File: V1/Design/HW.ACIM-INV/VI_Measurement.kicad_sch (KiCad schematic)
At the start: 59 parts, among them Q1 20V/1A, U12 OP-1CH, U15 OP-1CH, U16 OP-1CH, U2 OP-1CH, U4 CMP-1CH

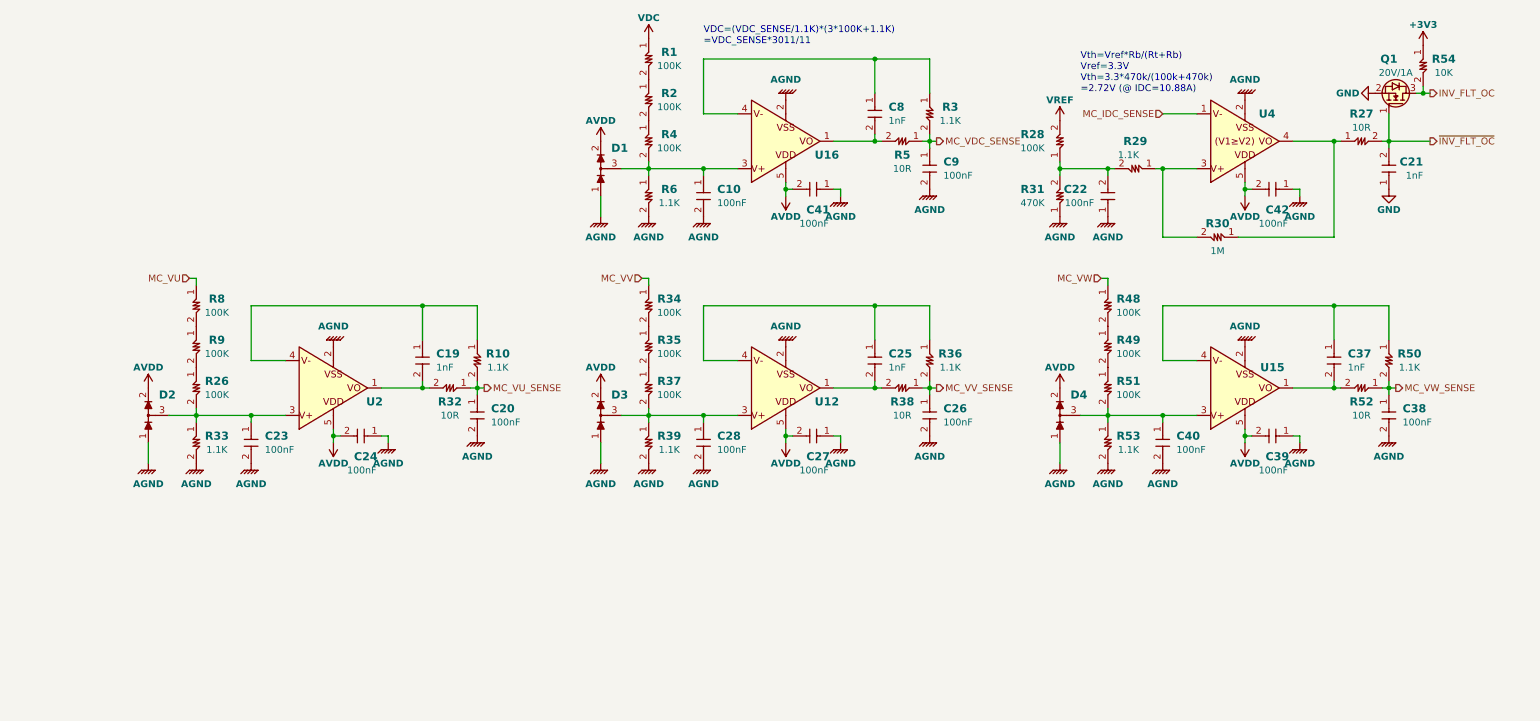
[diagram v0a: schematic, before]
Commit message: V1 schematic update 2
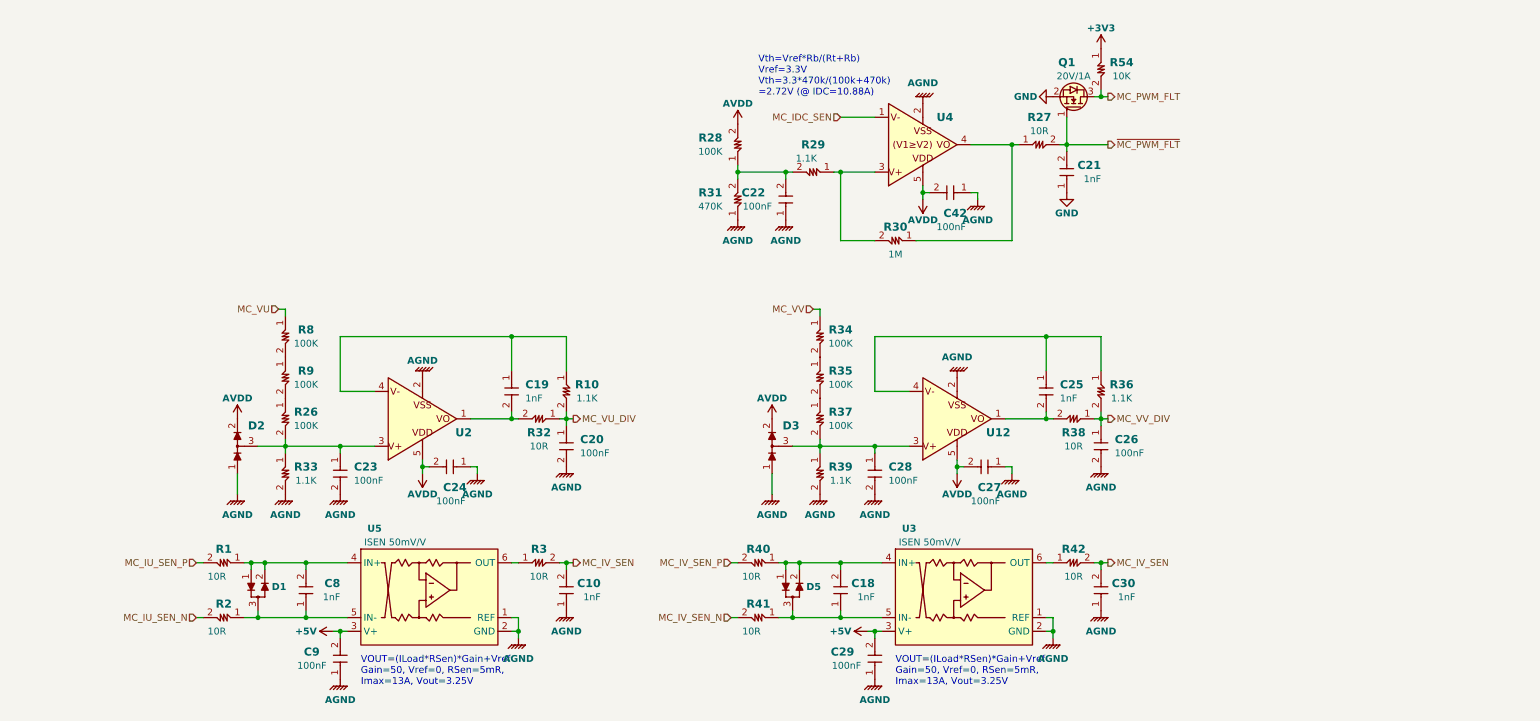
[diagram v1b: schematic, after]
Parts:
- removed C37: 1nF, SAMPI:CAP0603, symbol SAMPI:CERCAP
- removed C38, C39, C40, C41: 100nF, SAMPI:CAP0603, symbol SAMPI:CERCAP
- removed D1, D4: GP DIODE, SAMPI:SOT23, symbol SAMPI:DIODE_ARR2
- removed R4, R48, R49, R51: 100K, SAMPI:RES0603, symbol SAMPI:RES
- removed R5, R52: 10R, SAMPI:RES0603, symbol SAMPI:RES
- removed R50, R53, R6: 1.1K, SAMPI:RES0603, symbol SAMPI:RES
- removed U15, U16: OP-1CH, SAMPI:SOT353, symbol SAMPI:OPAMP-1CH
- added C18, C30: 1nF, SAMPI:CAP0603, symbol SAMPI:CERCAP
- added C29: 100nF, SAMPI:CAP0603, symbol SAMPI:CERCAP
- added D1, D5: GP DIODE, SAMPI:SOT23, symbol SAMPI:DIODE_ARR1
- added R40, R41, R42: 10R, SAMPI:RES0603, symbol SAMPI:RES
- added U3, U5: ISEN 50mV/V, SAMPI:SOT363, symbol SAMPI:ZXCT199Q
- C10: value 100nF -> 1nF; MNP CL10B104KB8NNNC -> CL10B102KB8NNNC; Unit Price 0.0146 -> 0.027
- R1, R2: value 100K -> 10R; MNP RC0603FR-07100KL -> RC0603FR-0710RL; Unit Price 0.019 -> 0.029
- R3: value 1.1K -> 10R; MNP AC0603FR-071K1L -> RC0603FR-0710RL; Unit Price 0.021 -> 0.029
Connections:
- net VDC is gone; now on an unnamed net: R1.1
- net VREF is gone; now on net AVDD: R28.2
- net AGND: now also C10.1, C9.1, C29.1, C30.1, U3.1 (REF), U3.2 (GND), U5.1 (REF), U5.2 (GND); no longer C10.2, C9.2
- net at C8.1: now also R2.1, D1.3 (COM), U5.5 (IN-); no longer R3.1
- net MC_IU_SEN_N: now reaches R2.2
- net at C8.2: now also D1.1 (A1), D1.2 (K2), U5.4 (IN+)
- net MC_IU_SEN_P: now reaches R1.2
- net MC_IU_SEN_P: no longer R2.1
- net INV_FLT_OC renamed MC_PWM_FLT
- net MC_IDC_SENSE renamed MC_IDC_SEN
- net MC_VDC_SENSE renamed MC_IV_SEN
- net MC_IV_SEN: now also C10.2, C30.2, R42.2; no longer C9.1
- net MC_VU_SENSE renamed MC_VU_DIV
- net MC_VV_SENSE renamed MC_VV_DIV
- net ~{INV_FLT_OC} renamed ~{MC_PWM_FLT}
- new net: C18.1, D5.3 (COM), R41.1, U3.5 (IN-)
- new net: R42.1, U3.6 (OUT)
- new net: C18.2, D5.1 (A1), D5.2 (K2), R40.1, U3.4 (IN+)
- new net: R3.1, U5.6 (OUT)
- new net +5V: C29.2, C9.2, U3.3 (V+), U5.3 (V+)
- new net MC_IV_SEN_N: R41.2
- new net MC_IV_SEN_P: R40.2
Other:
- note added: "VOUT=(ILoad*RSen)*Gain+Vref Gain=50, Vref=0, RSen=5mR, Imax=13A, Vout=3.25V"
- note removed: "VDC=(VDC_SENSE/1.1K)*(3*100K+1.1K) =VDC_SENSE*3011/11"
- moved on the sheet: C19, C20, C21, C22, C23, C24, C25, C26, C27, C28, C42, D2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

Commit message: V1 schematic update 3
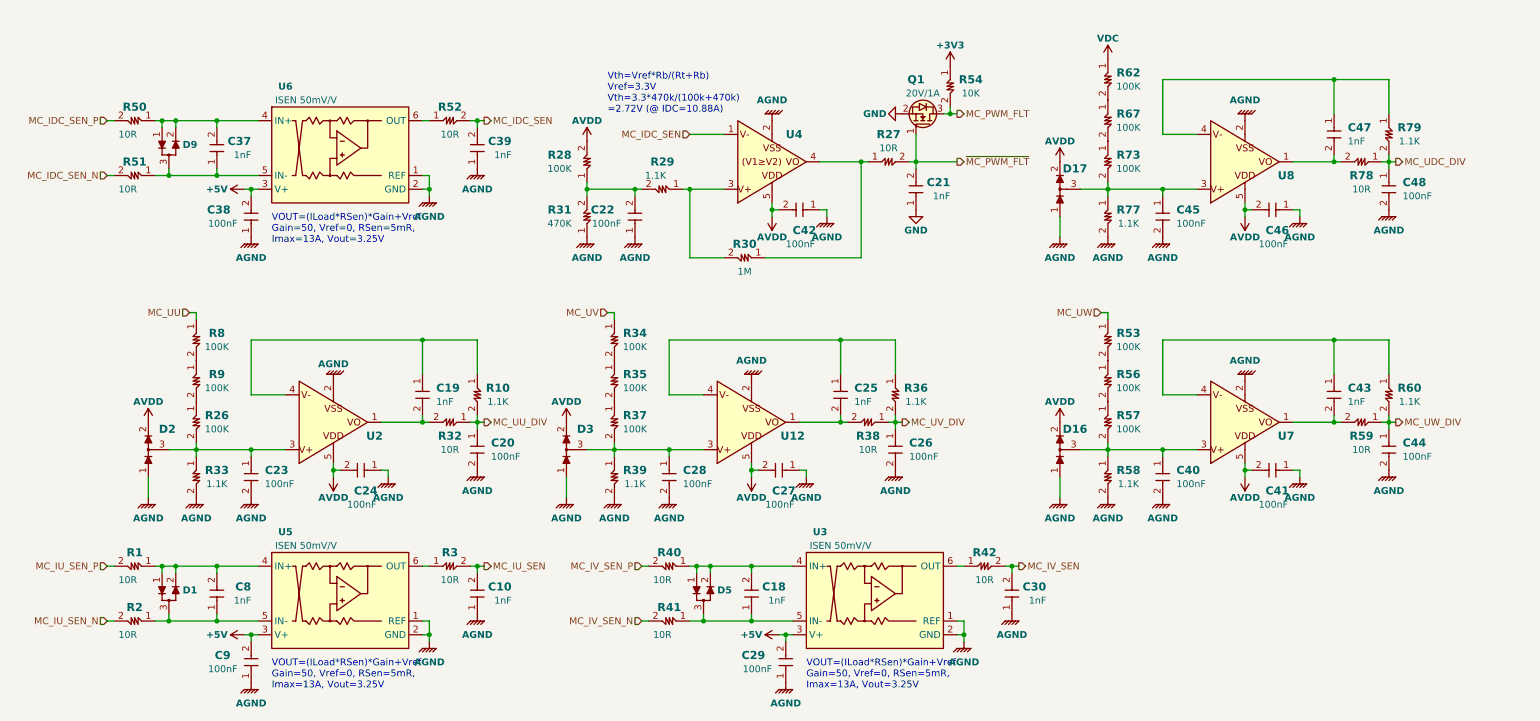
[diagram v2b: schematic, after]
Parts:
- added C37, C39, C43, C47: 1nF, SAMPI:CAP0603, symbol SAMPI:CERCAP
- added C38, C40, C41, C44, C45, C46, C48: 100nF, SAMPI:CAP0603, symbol SAMPI:CERCAP
- added D16, D17: GP DIODE, SAMPI:SOT23, symbol SAMPI:DIODE_ARR2
- added D9: GP DIODE, SAMPI:SOT23, symbol SAMPI:DIODE_ARR1
- added R50, R51, R52, R59, R78: 10R, SAMPI:RES0603, symbol SAMPI:RES
- added R53, R56, R57, R62, R67, R73: 100K, SAMPI:RES0603, symbol SAMPI:RES
- added R58, R60, R77, R79: 1.1K, SAMPI:RES0603, symbol SAMPI:RES
- added U6: ISEN 50mV/V, SAMPI:SOT363, symbol SAMPI:ZXCT199Q
- added U7, U8: OP-1CH, SAMPI:SOT353, symbol SAMPI:OPAMP-1CH
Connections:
- net +5V: now also C38.2, U6.3 (V+)
- net AGND: now also C38.1, C39.1, C40.2, C41.1, C44.2, C45.2, C46.1, C48.2, D16.1 (A1), D17.1 (A1), R58.2, R77.2, U6.1 (REF), U6.2 (GND), U7.2 (VSS), U8.2 (VSS)
- net AVDD: now also C41.2, C46.2, D16.2 (K2), D17.2 (K2), U7.5 (VDD), U8.5 (VDD)
- net MC_IDC_SEN: now also C39.2, R52.2
- net MC_IV_SEN: no longer C10.2, R3.2
- net MC_VU renamed MC_UU
- net MC_VU_DIV renamed MC_UU_DIV
- net MC_VV renamed MC_UV
- net MC_VV_DIV renamed MC_UV_DIV
- new net: R56.2, R57.1
- new net: C40.1, D16.3 (COM), R57.2, R58.1, U7.3 (VIN+)
- new net: C43.1, R60.1, U7.4 (VIN-)
- new net: C43.2, R59.2, U7.1 (VOUT)
- new net: C37.1, D9.3 (COM), R51.1, U6.5 (IN-)
- new net: R53.2, R56.1
- new net: C45.1, D17.3 (COM), R73.2, R77.1, U8.3 (VIN+)
- new net: C47.2, R78.2, U8.1 (VOUT)
- new net: C47.1, R79.1, U8.4 (VIN-)
- new net: C37.2, D9.1 (A1), D9.2 (K2), R50.1, U6.4 (IN+)
- new net: R67.2, R73.1
- new net: R62.2, R67.1
- new net: R52.1, U6.6 (OUT)
- new net MC_IDC_SEN_N: R51.2
- new net MC_IDC_SEN_P: R50.2
- new net MC_IU_SEN: C10.2, R3.2
- new net MC_UDC_DIV: C48.1, R78.1, R79.2
- new net MC_UW: R53.1
- new net MC_UW_DIV: C44.1, R59.1, R60.2
- new net VDC: R62.1
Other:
- moved on the sheet: C10, C18, C19, C20, C21, C22, C23, C24, C25, C26, C27, C28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

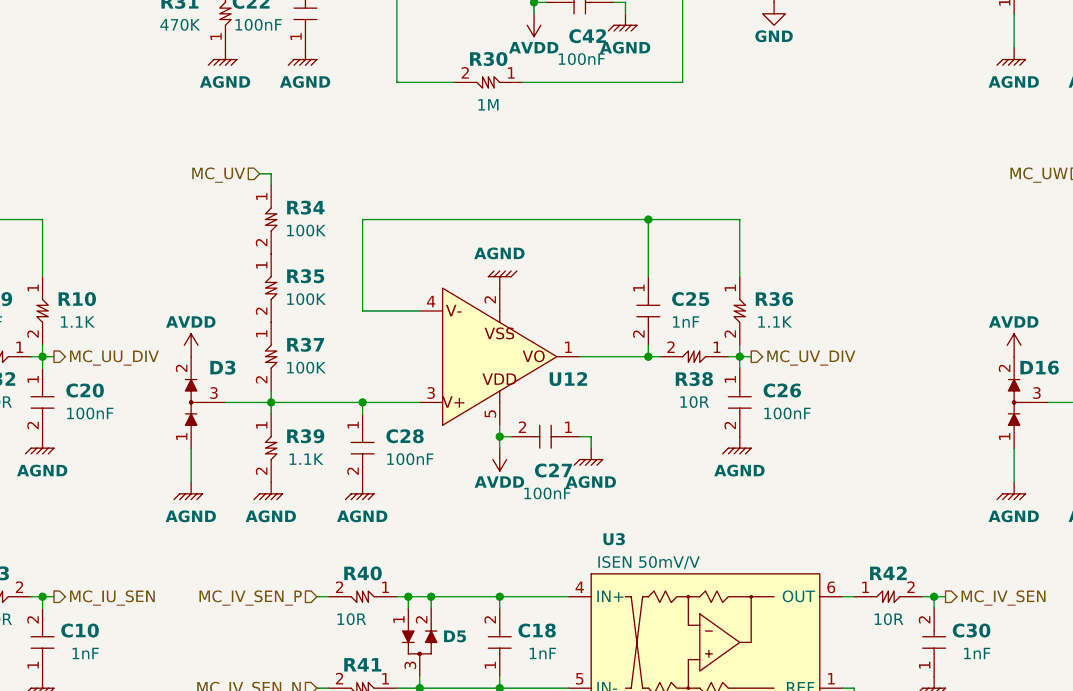
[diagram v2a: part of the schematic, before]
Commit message: V1 schematic update 5
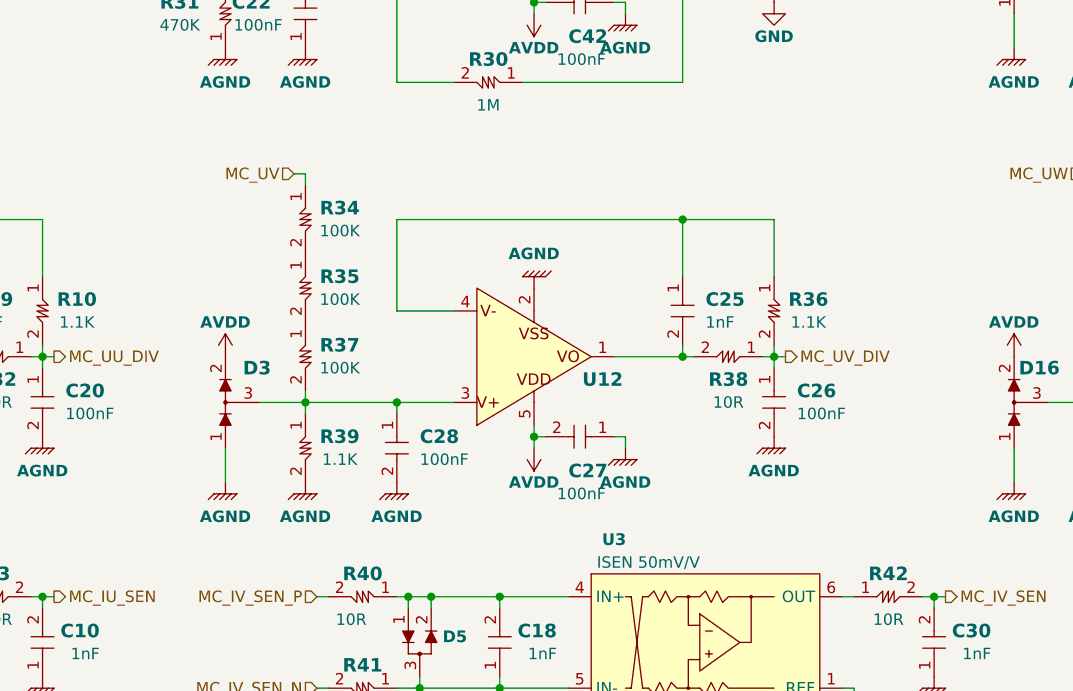
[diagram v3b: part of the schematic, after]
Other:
- moved on the sheet: C25, C26, C27, C28, D3, R34, R35, R36, R37, R38, R39, U12
